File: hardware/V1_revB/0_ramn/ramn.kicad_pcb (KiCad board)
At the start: 2 copper layers, 85.6 x 54 mm, 108 parts, among them J2 Screw_Terminal_01x03, J3 , J4 , J5 , J6 , P1 USB_C_Plug_USB2.0, U1 ATA6561-GAQW-N, U10 ATA6561-GAQW-N, U11 STM32L552/STM32L562, U12 NCV8163, U2 STM32L552/STM32L562, U3 NCV8163, U4 ATA6561-GAQW-N, U5 STM32L552/STM32L562, U6 NCV8163, U7 ATA6561-GAQW-N, U8 STM32L552/STM32L562, U9 NCV8163, Y1 NX3225GD-8MHZ-STD-CRA-3, Y2 NX3225GD-8MHZ-STD-CRA-3, Y3 NX3225GD-8MHZ-STD-CRA-3, Y4 NX3225GD-8MHZ-STD-CRA-3

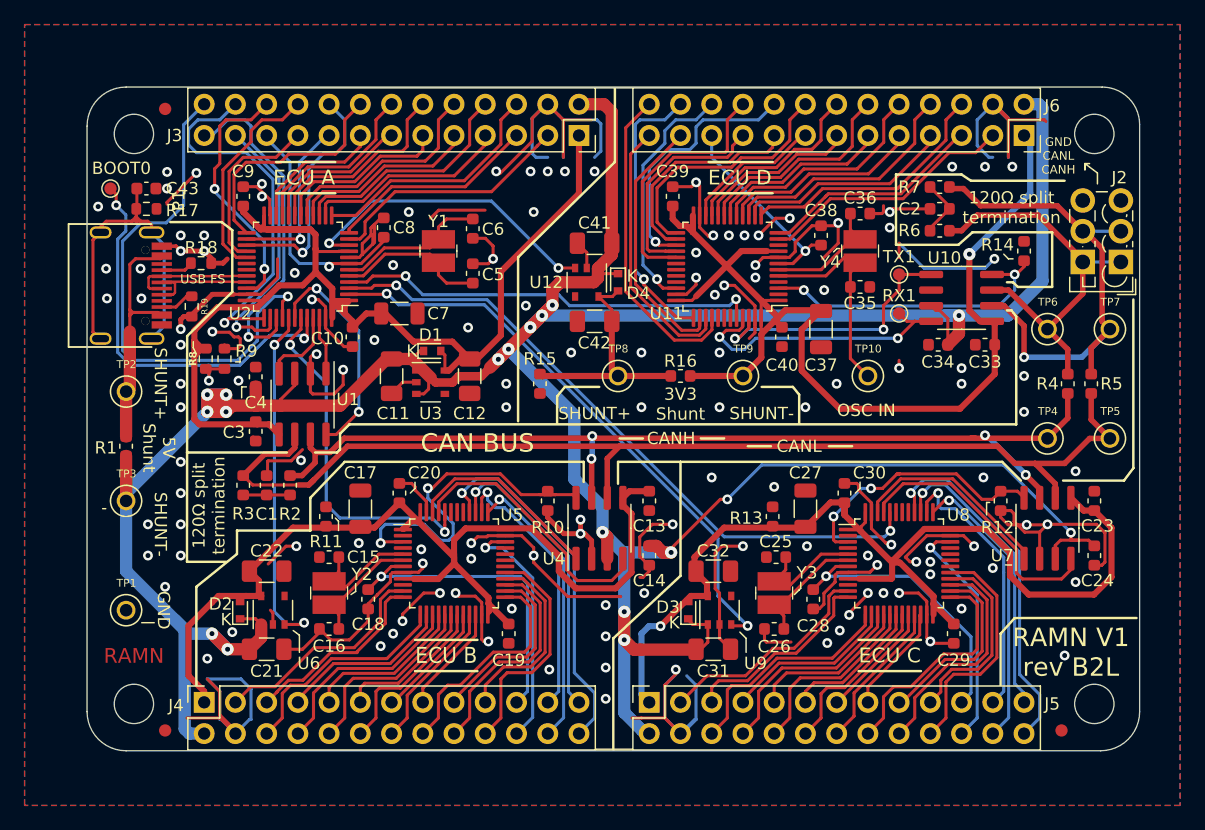
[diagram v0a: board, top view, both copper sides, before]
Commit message: fix: update files
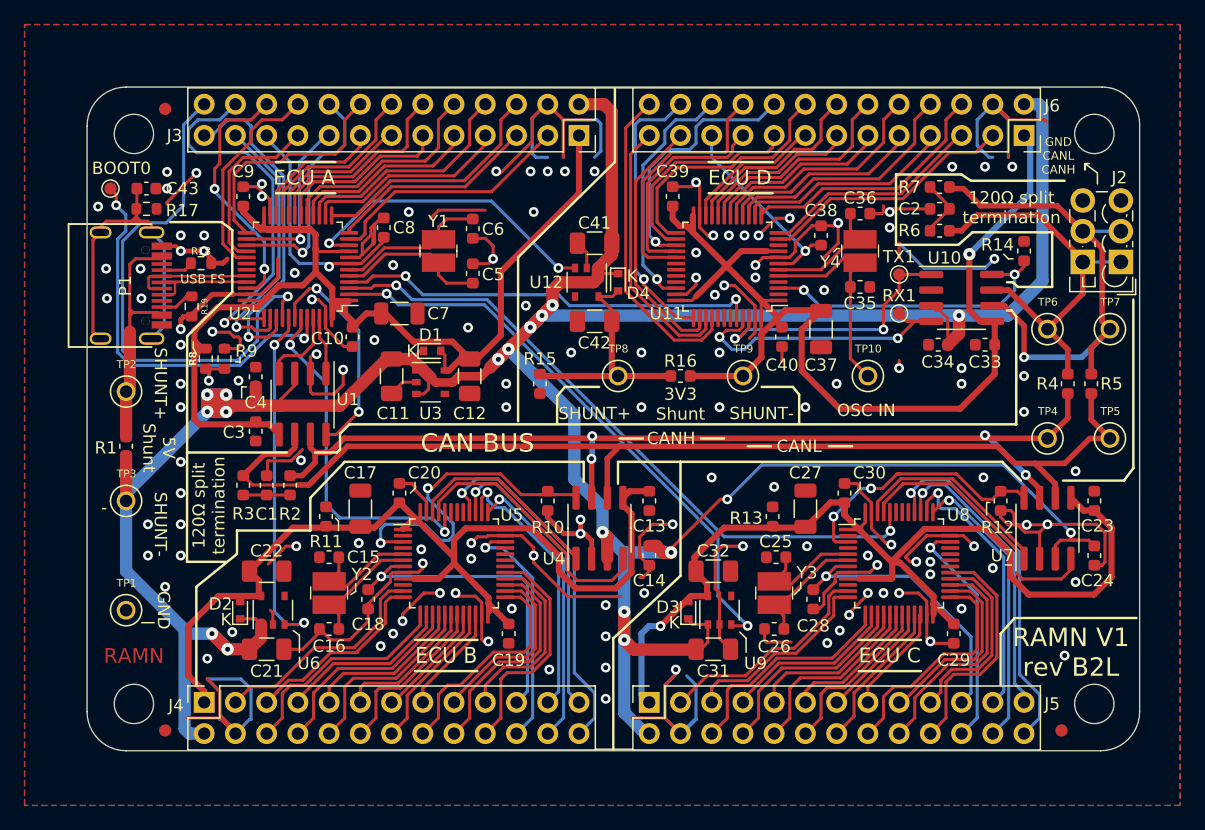
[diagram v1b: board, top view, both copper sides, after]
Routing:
- net +5V: track 304.8 -> 303.2 mm
- net GND: track 356.1 -> 357.4 mm
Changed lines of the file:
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@@
 			(sketchpadsonfab no)
 			(subtractmaskfromsilk no)
-			(outputformat 4)
+			(outputformat 1)
 			(mirror no)
 			(drillshape 0)
 			(scaleselection 1)
-			(outputdirectory "./CAD")
+			(outputdirectory "Main_Gebrer")
 		)
 	)
@@
 		)
 		(property ki_fp_filters "C_*")
-		(sheetname "Root")
+		(sheetname "Raíz")
 		(sheetfile "ramn.kicad_sch")
 		(attr smd)
@@
 		)
 		(property ki_fp_filters "R_*")
-		(sheetname "Root")
+		(sheetname "Raíz")
 		(sheetfile "ramn.kicad_sch")
 		(attr smd)
@@
 		)
 		(property ki_fp_filters "Pin* Test*")
-		(sheetname "Root")
+		(sheetname "Raíz")
 		(sheetfile "ramn.kicad_sch")
 		(attr through_hole)
@@
 		)
 		(property ki_fp_filters "R_*")
-		(sheetname "Root")
+		(sheetname "Raíz")
 		(sheetfile "ramn.kicad_sch")
 		(attr smd)
@@
 		)
 		(property ki_fp_filters "MountingHole*")
-		(sheetname "Root")
+		(sheetname "Raíz")
 		(sheetfile "ramn.kicad_sch")
 		(attr exclude_from_pos_files)
@@
 		)
 		(property ki_fp_filters "C_*")
-		(sheetname "Root")
+		(sheetname "Raíz")
 		(sheetfile "ramn.kicad_sch")
 		(attr smd)
@@
 		)
 		(property ki_fp_filters "R_*")
-		(sheetname "Root")
+		(sheetname "Raíz")
 		(sheetfile "ramn.kicad_sch")
 		(attr smd)
@@
 		)
 		(property ki_fp_filters "MountingHole*")
-		(sheetname "Root")
+		(sheetname "Raíz")
 		(sheetfile "ramn.kicad_sch")
 		(attr exclude_from_pos_files)
@@
 		)
 		(property ki_fp_filters "Pin* Test*")
-		(sheetname "Root")
+		(sheetname "Raíz")
 		(sheetfile "ramn.kicad_sch")
 		(attr through_hole)
@@
 		)
 		(property ki_fp_filters "Pin* Test*")
-		(sheetname "Root")
+		(sheetname "Raíz")
 		(sheetfile "ramn.kicad_sch")
 		(attr through_hole)
@@
 		)
 		(property ki_fp_filters "Pin* Test*")
-		(sheetname "Root")
+		(sheetname "Raíz")
 		(sheetfile "ramn.kicad_sch")
 		(attr through_hole)
@@
 		)
 		(property ki_fp_filters "MountingHole*")
-		(sheetname "Root")
+		(sheetname "Raíz")
 		(sheetfile "ramn.kicad_sch")
 		(attr exclude_from_pos_files)
@@
 		)
 		(property ki_fp_filters "Pin* Test*")
-		(sheetname "Root")
+		(sheetname "Raíz")
 		(sheetfile "ramn.kicad_sch")
 		(attr through_hole)
@@
 		)
 		(property ki_fp_filters "R_*")
-		(sheetname "Root")
+		(sheetname "Raíz")
 		(sheetfile "ramn.kicad_sch")
 		(attr smd)
@@
 		)
 		(property ki_fp_filters "R_*")
-		(sheetname "Root")
+		(sheetname "Raíz")
 		(sheetfile "ramn.kicad_sch")
 		(attr smd)
@@
 		)
 		(property ki_fp_filters "Pin* Test*")
-		(sheetname "Root")
+		(sheetname "Raíz")
 		(sheetfile "ramn.kicad_sch")
 		(attr through_hole)
@@
 		)
 		(property ki_fp_filters "Pin* Test*")
-		(sheetname "Root")
+		(sheetname "Raíz")
 		(sheetfile "ramn.kicad_sch")
 		(attr through_hole)
@@
 		)
 		(property ki_fp_filters "R_*")
-		(sheetname "Root")
+		(sheetname "Raíz")
 		(sheetfile "ramn.kicad_sch")
 		(attr smd)
@@
 		)
 		(property ki_fp_filters "MountingHole*")
-		(sheetname "Root")
+		(sheetname "Raíz")
 		(sheetfile "ramn.kicad_sch")
 		(clearance 1)
@@
 		)
 		(property ki_fp_filters "Fiducial*")
-		(sheetname "Root")
+		(sheetname "Raíz")
 		(sheetfile "ramn.kicad_sch")
 		(attr smd)
@@
 		)
 		(property ki_fp_filters "Fiducial*")
-		(sheetname "Root")
+		(sheetname "Raíz")
 		(sheetfile "ramn.kicad_sch")
 		(attr smd)
@@
 		)
 		(property ki_fp_filters "Fiducial*")
-		(sheetname "Root")
+		(sheetname "Raíz")
 		(sheetfile "ramn.kicad_sch")
 		(attr smd)
@@
 		)
 		(property ki_fp_filters "C_*")
-		(sheetname "Root")
+		(sheetname "Raíz")
 		(sheetfile "ramn.kicad_sch")
 		(attr smd)
@@
 		)
 		(property ki_fp_filters "R_*")
-		(sheetname "Root")
+		(sheetname "Raíz")
 		(sheetfile "ramn.kicad_sch")
 		(attr smd)
@@
 		)
 		(property ki_fp_filters "TerminalBlock*:*")
-		(sheetname "Root")
+		(sheetname "Raíz")
 		(sheetfile "ramn.kicad_sch")
 		(attr through_hole)
@@
 		)
 		(property ki_fp_filters "R_*")
-		(sheetname "Root")
+		(sheetname "Raíz")
 		(sheetfile "ramn.kicad_sch")
 		(attr smd)
@@
 		)
 		(property ki_fp_filters "R_*")
-		(sheetname "Root")
+		(sheetname "Raíz")
 		(sheetfile "ramn.kicad_sch")
 		(attr smd)
@@
 		(tags "resistor")
 		(property "Reference" "R18"
-			(at -0.01 1.26 0)
+			(at 0 0.97 0)
 			(layer "F.SilkS")
 			(effects
 				(font
-					(size 1 1)
+					(size 0.6 0.6)
 					(thickness 0.15)
 				)
@@
 		)
 		(property ki_fp_filters "R_*")
-		(sheetname "Root")
+		(sheetname "Raíz")
 		(sheetfile "ramn.kicad_sch")
 		(attr smd)
@@
 		(at 45.89 59.32 -90)
 		(property "Reference" "P1"
-			(at -6.9 -2.2 90)
+			(at 0.02 2.14 90)
 			(layer "F.SilkS")
 			(effects
@@
 		)
 		(property ki_fp_filters "USB*C*Plug*")
-		(sheetname "Root")
+		(sheetname "Raíz")
 		(sheetfile "ramn.kicad_sch")
 		(attr through_hole)
@@
 	)
 	(segment
+		(start 97.155 64.2875)
+		(end 97.155 65.505)
+		(width 0.25)
+		(layer "F.Cu")
+		(net 1)
+	)
+	(segment
 		(start 49.53 50.165)
 		(end 47.1425 52.5525)
@@
 	)
 	(segment
+		(start 97.155 65.505)
+		(end 97.14 65.52)
+		(width 0.25)
+		(layer "F.Cu")
+		(net 1)
+	)
+	(segment
 		(start 114.3 44.577)
 		(end 114.427 44.577)
@@
 	)
 	(segment
-		(start 47.752 86.487)
-		(end 48.895 87.63)
-		(width 1)
-		(layer "B.Cu")
-		(net 3)
-	)
-	(segment
 		(start 74.909499 64.495499)
 		(end 80.264 69.85)
@@
 	)
 	(segment
-		(start 73.025 84.455)
-		(end 73.28501 84.71501)
-		(width 0.25)
-		(layer "F.Cu")
-		(net 79)
-	)
-	(segment
 		(start 57.3875 79.0075)
 		(end 62.865 79.0075)
@@
 	)
 	(segment
-		(start 115.189001 82.676999)
-		(end 115.189 82.677)
-		(width 0.25)
-		(layer "B.Cu")
-		(net 128)
-	)
-	(segment
 		(start 115.189 81.412394)
 		(end 111.246606 77.47)
@@
 	)
 	(segment
-		(start 112.53701 71.73999)
-		(end 113.39599 71.73999)
-		(width 0.45)
-		(layer "F.Cu")
-		(net 154)
-	)
-	(segment
 		(start 113.538 71.373999)
 		(end 113.665 71.500999)
@@
 	)
 	(segment
-		(start 81.42201 71.73999)
-		(end 112.53701 71.73999)
-		(width 0.45)
-		(layer "F.Cu")
-		(net 154)
-	)
-	(segment
 		(start 57.15 74.7775)
 		(end 58.128 74.7775)
@@
 	)
 	(segment
-		(start 112.53701 71.73999)
-		(end 112.89251 71.73999)
+		(start 61.5552 71.73999)
+		(end 81.42201 71.73999)
 		(width 0.45)
 		(layer "F.Cu")
@@
 	)
 	(segment
-		(start 61.5552 71.73999)
-		(end 81.42201 71.73999)
+		(start 81.42201 71.73999)
+		(end 113.39599 71.73999)
 		(width 0.45)
 		(layer "F.Cu")
